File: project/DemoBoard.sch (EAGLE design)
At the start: 51 parts, among them J1 SAMTEC-MMS-105-02-X-SVJ, J4 10104111-0001LF, U1 SN74LVC2T45YZPR, U2 STM32F207ZGT6, U3 SN74LVC2T45YZPR, U4 SN74LVC2T45YZPR, Y1 SIT1602BI-23-18E-33.333300G, Y2 SIT1602BI-23-18E-33.333300G, Y3 SIT1602BI-23-18E-33.333300G

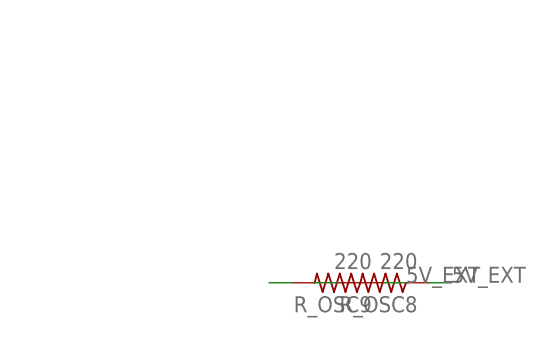
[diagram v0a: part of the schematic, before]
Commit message: Add files via upload
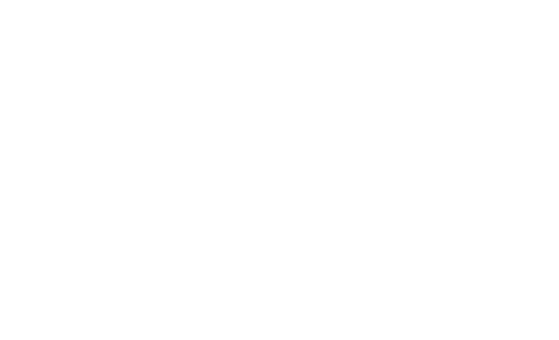
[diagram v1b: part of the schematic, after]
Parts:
- removed R_OSC8, R_OSC9: 220, rcl:R-US_R0805
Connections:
- removed net N$26: R_OSC8.1
- removed net N$27: R_OSC9.1
- removed net VCC1: R_OSC8.2
- removed net VCC2: R_OSC9.2
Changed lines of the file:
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@@
 <part name="U2" library="STM32F207ZGT6" deviceset="STM32F207ZGT6" device=""/>
 <part name="R_OSC7" library="rcl" library_urn="urn:adsk.eagle:library:334" deviceset="R-US_" device="R0805" package3d_urn="urn:adsk.eagle:package:23553/2" value="330"/>
-<part name="R_OSC8" library="rcl" library_urn="urn:adsk.eagle:library:334" deviceset="R-US_" device="R0805" package3d_urn="urn:adsk.eagle:package:23553/2" value="220"/>
-<part name="R_OSC9" library="rcl" library_urn="urn:adsk.eagle:library:334" deviceset="R-US_" device="R0805" package3d_urn="urn:adsk.eagle:package:23553/2" value="220"/>
 <part name="R_OSC10" library="rcl" library_urn="urn:adsk.eagle:library:334" deviceset="R-US_" device="R0805" package3d_urn="urn:adsk.eagle:package:23553/2" value="330"/>
 <part name="U1" library="SN74LVC2T45YZPR" deviceset="SN74LVC2T45YZPR" device=""/>
@@
 <attribute name="NAME" x="367.03" y="-377.4186" size="1.778" layer="95" rot="R180"/>
 <attribute name="VALUE" x="367.03" y="-372.618" size="1.778" layer="96" rot="R180"/>
-</instance>
-<instance part="R_OSC8" gate="G$1" x="541.02" y="-619.76" smashed="yes" rot="R180">
-<attribute name="NAME" x="544.83" y="-621.2586" size="1.778" layer="95" rot="R180"/>
-<attribute name="VALUE" x="544.83" y="-616.458" size="1.778" layer="96" rot="R180"/>
-</instance>
-<instance part="R_OSC9" gate="G$1" x="535.94" y="-619.76" smashed="yes" rot="R180">
-<attribute name="NAME" x="539.75" y="-621.2586" size="1.778" layer="95" rot="R180"/>
-<attribute name="VALUE" x="539.75" y="-616.458" size="1.778" layer="96" rot="R180"/>
 </instance>
 <instance part="R_OSC10" gate="G$1" x="363.22" y="-391.16" smashed="yes" rot="R180">
@@
 </segment>
 <segment>
-<label x="548.64" y="-619.76" size="1.778" layer="95"/>
-</segment>
-<segment>
-<label x="543.56" y="-619.76" size="1.778" layer="95"/>
-</segment>
-<segment>
 <label x="152.4" y="-10.16" size="1.778" layer="95" rot="R90"/>
 </segment>
@@
 </segment>
 </net>
-<net name="VCC1" class="0">
-<segment>
-<wire x1="533.4" y1="-619.76" x2="535.94" y2="-619.76" width="0.1524" layer="91"/>
-<pinref part="R_OSC8" gate="G$1" pin="2"/>
-</segment>
-</net>
-<net name="N$26" class="0">
-<segment>
-<pinref part="R_OSC8" gate="G$1" pin="1"/>
-<wire x1="546.1" y1="-619.76" x2="548.64" y2="-619.76" width="0.1524" layer="91"/>
-</segment>
-</net>
-<net name="VCC2" class="0">
-<segment>
-<wire x1="528.32" y1="-619.76" x2="530.86" y2="-619.76" width="0.1524" layer="91"/>
-<pinref part="R_OSC9" gate="G$1" pin="2"/>
-</segment>
-</net>
-<net name="N$27" class="0">
-<segment>
-<pinref part="R_OSC9" gate="G$1" pin="1"/>
-<wire x1="541.02" y1="-619.76" x2="543.56" y2="-619.76" width="0.1524" layer="91"/>
-</segment>
-</net>
